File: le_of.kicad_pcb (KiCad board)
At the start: 2 copper layers, 20 parts, among them IC1 LTC3631EMS8E-3.3#PBF, J1 ST_Link_Connector, J2 ATM13-12PA-R008, U2 STM32G0B1REI6N

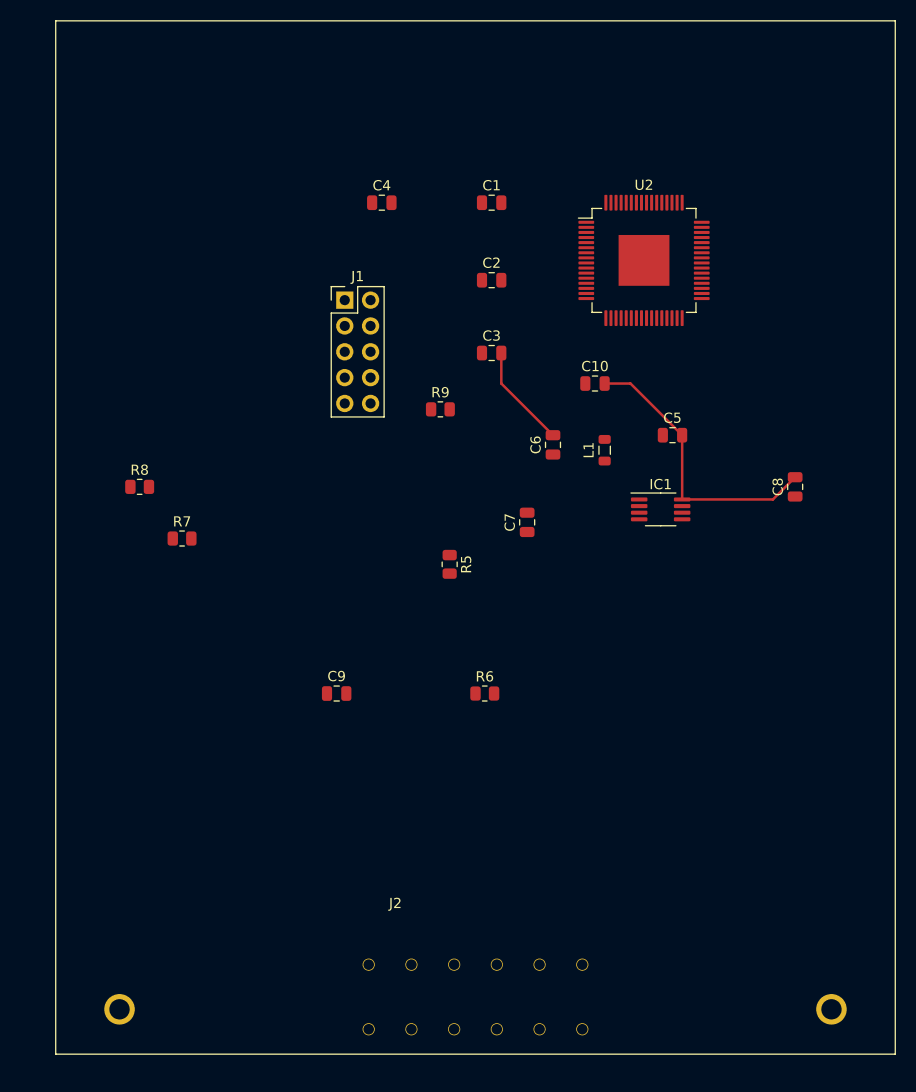
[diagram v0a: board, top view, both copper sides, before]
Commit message: added bunch
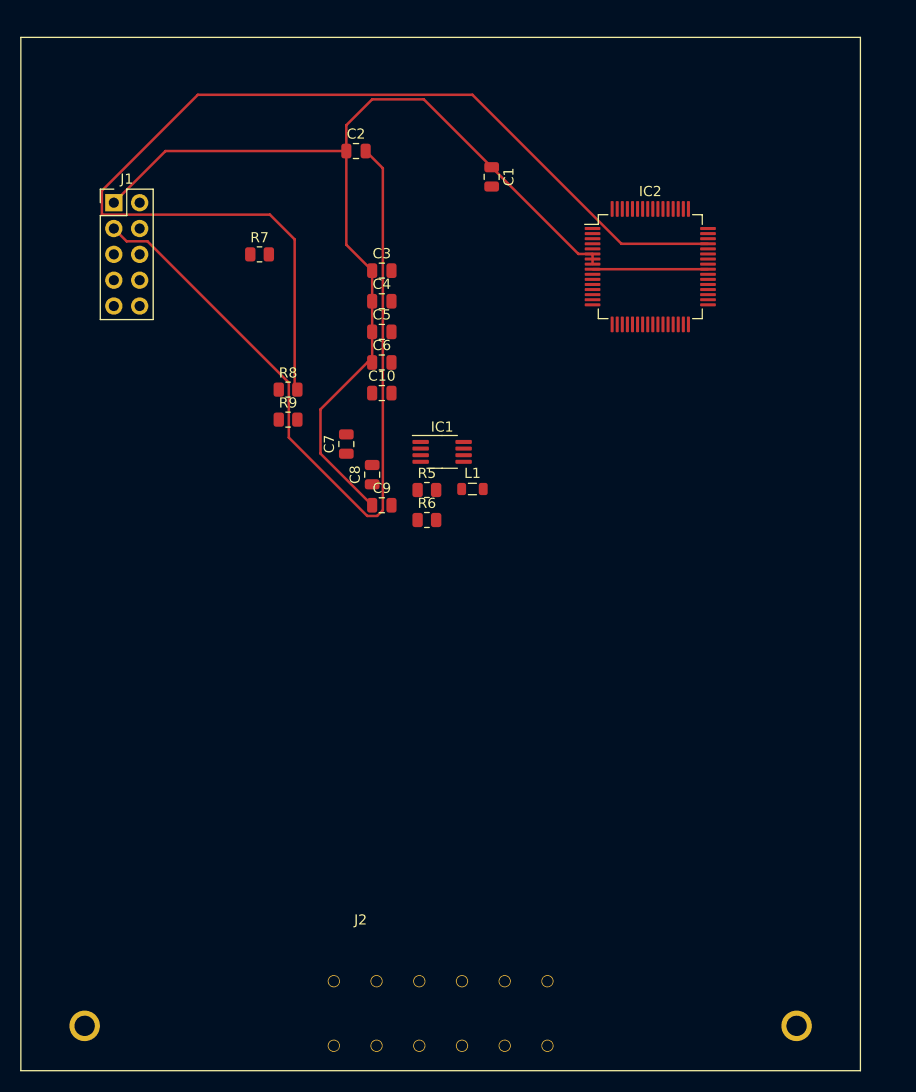
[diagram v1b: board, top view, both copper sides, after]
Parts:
- removed U2: STM32G0B1REI6N, Package_QFP:LQFP-64-1EP_10x10mm_P0.5mm_EP5x5mm
- added IC2: STM32G0B1RET6N, Package_QFP:LQFP-64_10x10mm_P0.5mm, F.Cu at (149.3, 64.7)
- C1, C2: value 100n0 -> 4u7
- C3, C4: value 4u7 -> 100n0
- moved C8 41.6 mm to (121.9, 85.2)
- moved C5 30.3 mm to (122.9, 71.1)
- moved R7 29.0 mm to (110.8, 63.5)
- moved J1 24.6 mm to (96.5, 58.4)
- moved IC1 22.2 mm to (128.8, 82.9)
- moved C10 21.0 mm to (122.9, 77.1)
- moved C7 19.4 mm to (119.4, 82.2)
- moved C9 19.0 mm to (122.9, 88.2)
- moved C6 18.7 mm to (122.9, 74.1), turned to 0 degrees
- moved C2 18.4 mm to (120.3, 53.3)
- moved R6 18.0 mm to (127.3, 89.6)
- moved R8 17.4 mm to (113.7, 76.8)
- moved R9 15.0 mm to (113.7, 79.8)
- moved L1 13.5 mm to (131.8, 86.6), turned to 0 degrees
- moved C3 13.5 mm to (122.9, 65.1)
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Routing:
- net /microprocessor/SWDIO: track 0.00 -> 106.1 mm
- net +3V3: track 0.00 -> 100.4 mm
- net GND: track 38.2 -> 88.9 mm
